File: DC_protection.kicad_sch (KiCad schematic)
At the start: 15 parts

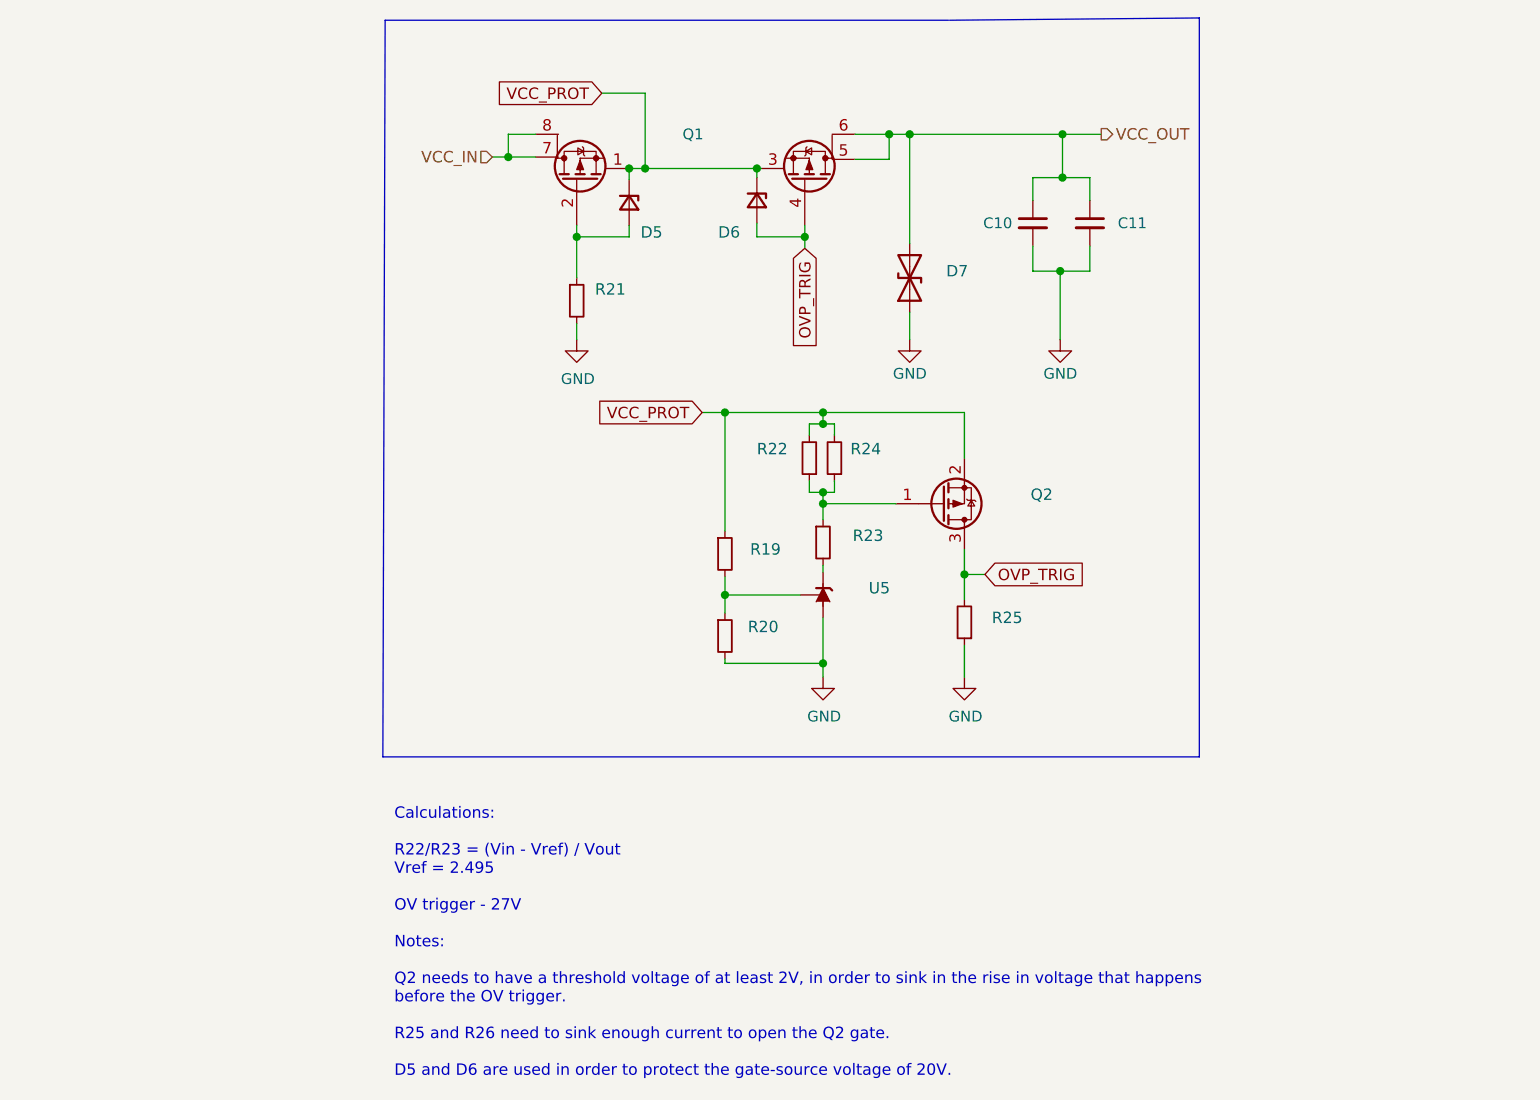
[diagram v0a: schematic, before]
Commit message: Exported updated gerbers
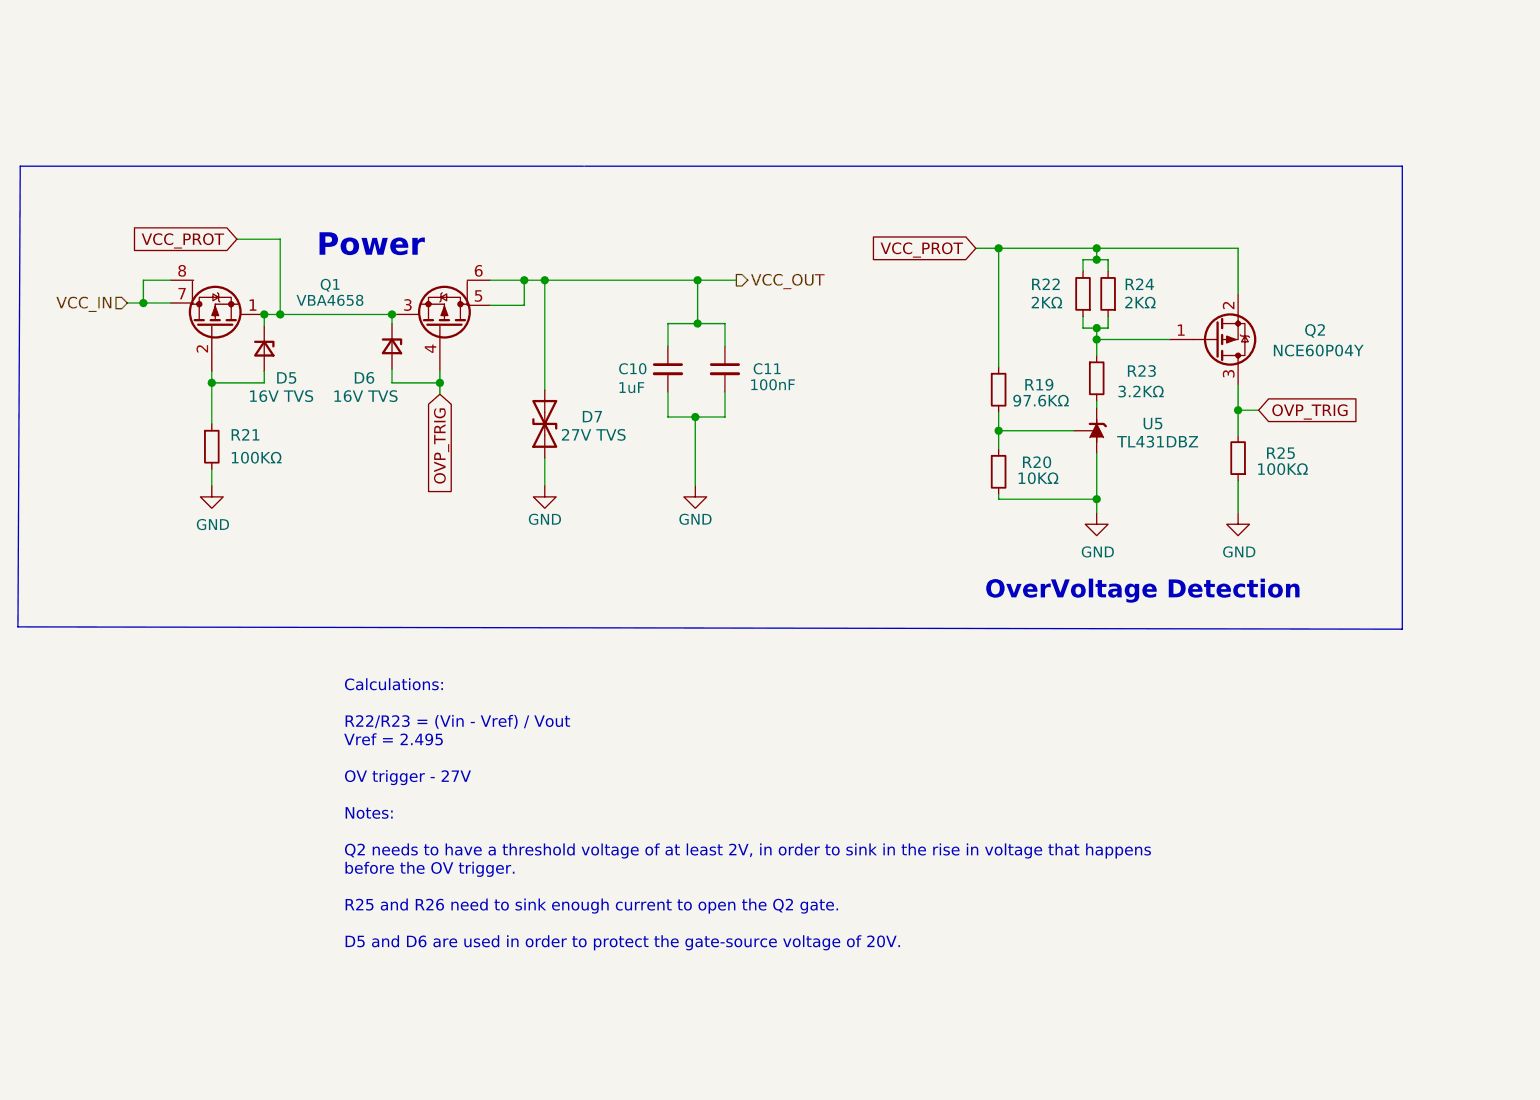
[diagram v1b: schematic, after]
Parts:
- C10: value (none) -> 1uF; footprint (none) -> Capacitor_SMD:C_0805_2012Metric
- C11: value (none) -> 100nF; footprint (none) -> Capacitor_SMD:C_0603_1608Metric
- D5, D6: value (none) -> 16V TVS
- D7: value (none) -> 27V TVS; footprint (none) -> Diode_SMD:D_SOD-523
- Q1: value ~ -> VBA4658; footprint (none) -> Package_SO:SO-8_3.9x4.9mm_P1.27mm
- Q2: value (none) -> NCE60P04Y; footprint (none) -> Package_TO_SOT_SMD:SOT-23
- R19: value (none) -> 97.6KΩ; footprint (none) -> Resistor_SMD:R_0603_1608Metric
- R20: value (none) -> 10KΩ; footprint (none) -> Resistor_SMD:R_0603_1608Metric
- R21, R25: value (none) -> 100KΩ; footprint (none) -> Resistor_SMD:R_0603_1608Metric
- R22, R24: value (none) -> 2KΩ; footprint (none) -> Resistor_SMD:R_0603_1608Metric
- R23: value (none) -> 3.2KΩ; footprint (none) -> Resistor_SMD:R_0603_1608Metric
- U5: value (none) -> TL431DBZ
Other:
- note added: "OverVoltage Detection"
- note added: "Power"
- moved on the sheet: C10, C11, D5, D6, D7, Q1, Q2, R19, R20, R21, R22, R23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
